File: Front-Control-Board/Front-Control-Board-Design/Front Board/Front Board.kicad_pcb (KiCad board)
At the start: 2 copper layers, 26 parts, among them J1 Conn_01x08, J2 Conn_01x23, Q1 2N7002, U1 MAX33054EASA+T, U2 TS2940CP33 ROG, U3 ESP32-DevKitC

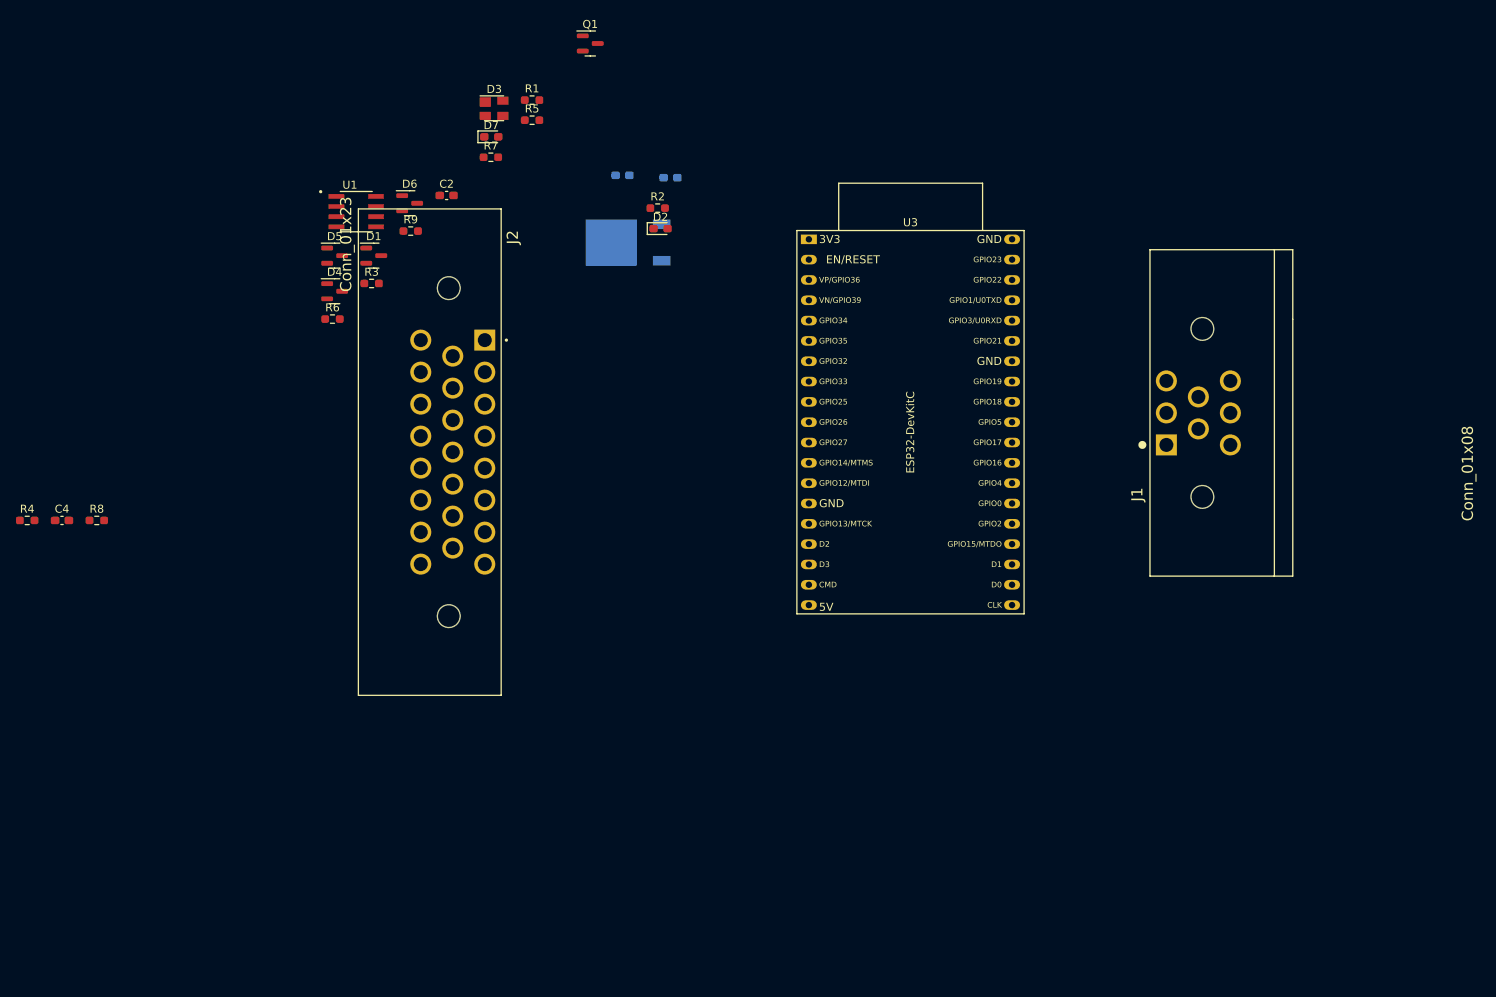
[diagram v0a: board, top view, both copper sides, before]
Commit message: Front Board V1
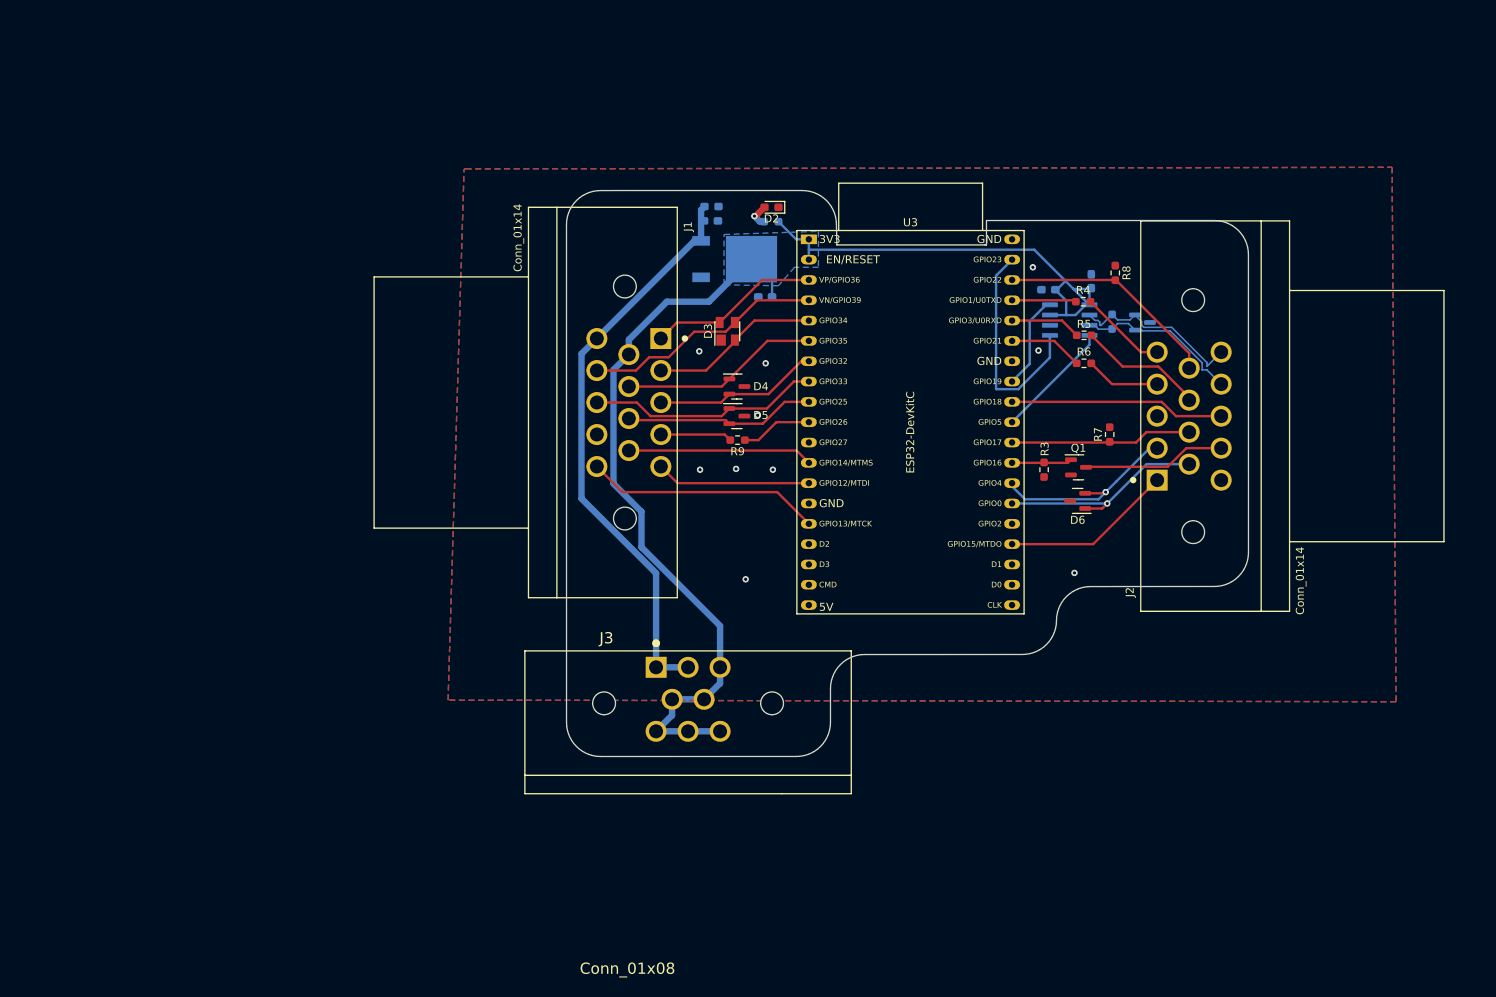
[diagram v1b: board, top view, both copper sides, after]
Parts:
- added J3: Conn_01x08, AERO_Footprints:TE_1-776280-1_8pin_Horizontal, F.Cu at (166.7, 136.1)
- C2, C4, D1, D7, R1, R2, U1: moved to B.Cu
- J1: value Conn_01x08 -> Conn_01x14; footprint AERO_Footprints:TE_1-776280-1_8pin_Horizontal -> AERO_Footprints:TE_1-776266-1_14pin_Horizontal
- J2: value Conn_01x23 -> Conn_01x14; footprint AERO_Footprints:TE_1-770669-1_23pin_Horizontal -> AERO_Footprints:TE_1-776266-1_14pin_Horizontal
- moved R4 134.8 mm to (216.1, 85.9)
- moved R8 131.0 mm to (220.1, 82.3), turned to -90 degrees
- moved C4 126.6 mm to (211.7, 84.4), turned to 180 degrees
- moved D1 96.5 mm to (223.5, 88.5)
- moved R6 94.1 mm to (216.2, 93.6)
- moved D6 91.4 mm to (215.4, 110.8), turned to 180 degrees
- moved U1 90.2 mm to (214.4, 88.2)
- moved J2 88.6 mm to (229.3, 100.2), turned to 90 degrees
- moved R3 87.2 mm to (211.2, 106.9), turned to -90 degrees
- moved R7 84.8 mm to (219.4, 102.5), turned to 90 degrees
- moved Q1 80.8 mm to (215.5, 106.6)
- moved R1 77.6 mm to (219.7, 88.4), turned to 90 degrees
- moved R5 74.1 mm to (216.2, 90.1), turned to 180 degrees
- moved J1 71.7 mm to (159.3, 98.5), turned to -90 degrees
- moved C3 54.2 mm to (217.1, 83.3), turned to 90 degrees
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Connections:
- D1 pad 1: /CAN_N -> /CAN_P
- D1 pad 2: /CAN_P -> /CAN_N
- D3 pad 1: unconnected-(D3-Pad1) -> GND
- D3 pad 2: /R_wheel -> /L_sus
- D3 pad 4: /L_sus -> /R_wheel
- J1 pad 1: GND -> /R_wheel
- J1 pad 2: /LORA NSS -> /L_sus
- J1 pad 3: /LORA Reset -> /stearing
- J1 pad 4: /LORA_RX -> /WCB_status
- J1 pad 5: /LORA_TX -> /LORA_MISO
- J1 pad 6: /pedal_0 -> VDD
- J1 pad 7: /Brake_0 -> /R_sus
- J1 pad 8: /Brake_1 -> /pedal_1
- J2 pad 1: /RTD_ind_out -> /LoRa_CS
- J2 pad 10: /RTD_led -> unconnected-(J2-Pad10)
- J2 pad 11: /stearing -> /RTD_ind_out
- J2 pad 12: /L_wheel -> unconnected-(J2-Pad12)
- J2 pad 13: /L_sus -> /CAN_P
- J2 pad 14: VDD -> /CAN_N
- J2 pad 2: /IMD_led -> /Brake_0
- J2 pad 3: /RTD_bttn -> unconnected-(J2-Pad3)
- J2 pad 4: /pedal_1 -> /RTD_led
- J2 pad 5: /R_wheel -> /AMS_Led
- J2 pad 6: /R_sus -> /Brake_1
- J2 pad 7: unconnected-(J2-Pad7) -> /RTD_bttn
- J2 pad 8: /CAN_N -> /IMD_led
- J2 pad 9: /AMS_Led -> /LORA Reset
- U1 pad 8: GND -> /CAN_CS
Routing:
- net VDD: track 0.00 -> 154.8 mm
- net +12V: track 0.00 -> 72.3 mm
- net /L_wheel: track 0.00 -> 30.1 mm
- net /Laura_MOSI: track 0.00 -> 29.5 mm
- net /pedal_0: track 0.00 -> 29.0 mm
- net /CAN_MOSI: track 0.00 -> 28.1 mm
- net /LORA Reset: track 0.00 -> 27.8 mm
- net /Brake_1: track 0.00 -> 27.2 mm, vias 0 -> 1
- net /CAN_SCK: track 0.00 -> 26.9 mm
- net /R_sus: track 0.00 -> 24.9 mm
- net /Brake_0: track 0.00 -> 24.5 mm, vias 0 -> 1
- net /pedal_1: track 0.00 -> 23.9 mm
- net /LORA_SCK: track 0.00 -> 23.1 mm
- net /RTD_bttn: track 0.00 -> 22.7 mm
- net /CAN_N: track 0.00 -> 22.3 mm
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- added copper zone on B.Cu, net GND
- added copper zone on F.Cu, net GND
- added copper zone on B.Cu, net VDD
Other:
- board outline added: 85.2 x 70.7 mm
